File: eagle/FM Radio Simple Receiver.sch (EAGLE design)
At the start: 14 parts, among them T1 2N2222, T2 2N2222

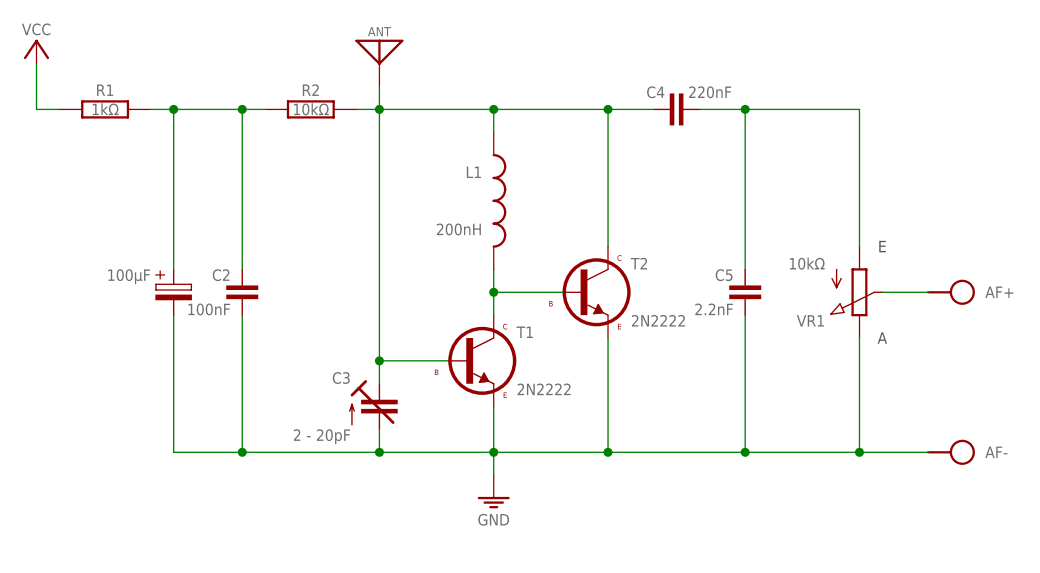
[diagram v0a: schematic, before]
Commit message: ...
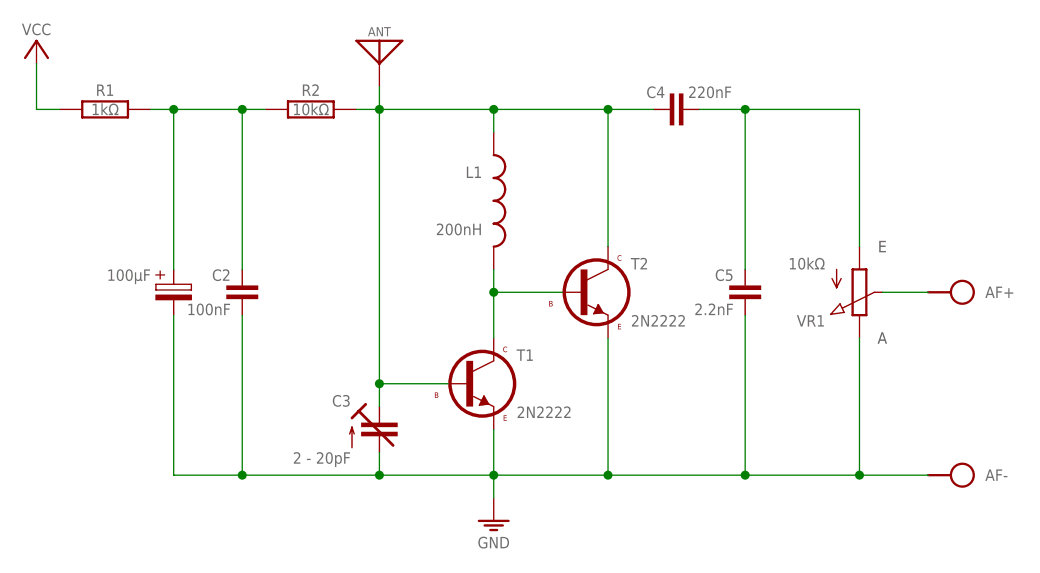
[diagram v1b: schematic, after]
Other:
- moved on the sheet: AF-, C3, T1
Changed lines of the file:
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@@
 </plain>
 <instances>
-<instance part="T1" gate="G$1" x="38.1" y="60.96"/>
-<instance part="C3" gate="1" x="27.94" y="55.88"/>
+<instance part="T1" gate="G$1" x="38.1" y="58.42"/>
+<instance part="C3" gate="1" x="27.94" y="53.34"/>
 <instance part="L1" gate="1" x="40.64" y="78.74"/>
 <instance part="T2" gate="G$1" x="50.8" y="68.58"/>
@@
 <instance part="VR1" gate="1" x="81.28" y="68.58" rot="MR180"/>
 <instance part="R2" gate="1" x="20.32" y="88.9"/>
-<instance part="AF" gate="-" x="88.9" y="50.8" rot="R180"/>
+<instance part="AF" gate="-" x="88.9" y="48.26" rot="R180"/>
 <instance part="AF" gate="+" x="88.9" y="68.58" rot="R180"/>
 <instance part="BAT" gate="1" x="-10.16" y="93.98"/>
-<instance part="BAT" gate="2" x="40.64" y="48.26"/>
+<instance part="BAT" gate="2" x="40.64" y="45.72"/>
 <instance part="ANT" gate="ANT" x="27.94" y="91.44"/>
 <instance part="C5" gate="1" x="68.58" y="68.58"/>
@@
 <pinref part="C3" gate="1" pin="E"/>
 <pinref part="T1" gate="G$1" pin="B"/>
-<wire x1="35.56" y1="60.96" x2="27.94" y2="60.96" width="0.1524" layer="91"/>
-<wire x1="27.94" y1="60.96" x2="27.94" y2="58.42" width="0.1524" layer="91"/>
-<wire x1="27.94" y1="60.96" x2="27.94" y2="88.9" width="0.1524" layer="91"/>
-<junction x="27.94" y="60.96"/>
+<wire x1="35.56" y1="58.42" x2="27.94" y2="58.42" width="0.1524" layer="91"/>
+<wire x1="27.94" y1="58.42" x2="27.94" y2="55.88" width="0.1524" layer="91"/>
+<wire x1="27.94" y1="58.42" x2="27.94" y2="88.9" width="0.1524" layer="91"/>
+<junction x="27.94" y="58.42"/>
 <pinref part="C4" gate="1" pin="1"/>
 <pinref part="L1" gate="1" pin="1"/>
@@
 <wire x1="40.64" y1="71.12" x2="40.64" y2="68.58" width="0.1524" layer="91"/>
 <pinref part="T2" gate="G$1" pin="B"/>
-<wire x1="40.64" y1="68.58" x2="40.64" y2="66.04" width="0.1524" layer="91"/>
+<wire x1="40.64" y1="68.58" x2="40.64" y2="63.5" width="0.1524" layer="91"/>
 <wire x1="48.26" y1="68.58" x2="40.64" y2="68.58" width="0.1524" layer="91"/>
 <junction x="40.64" y="68.58"/>
@@
 <segment>
 <pinref part="BAT" gate="2" pin="GND"/>
-<wire x1="40.64" y1="50.8" x2="40.64" y2="48.26" width="0.1524" layer="91"/>
+<wire x1="40.64" y1="48.26" x2="40.64" y2="45.72" width="0.1524" layer="91"/>
 <pinref part="VR1" gate="1" pin="E"/>
-<wire x1="81.28" y1="50.8" x2="81.28" y2="63.5" width="0.1524" layer="91"/>
+<wire x1="81.28" y1="48.26" x2="81.28" y2="63.5" width="0.1524" layer="91"/>
 <pinref part="AF" gate="-" pin="P$1"/>
-<wire x1="88.9" y1="50.8" x2="81.28" y2="50.8" width="0.1524" layer="91"/>
+<wire x1="88.9" y1="48.26" x2="81.28" y2="48.26" width="0.1524" layer="91"/>
 <pinref part="T1" gate="G$1" pin="E"/>
-<wire x1="40.64" y1="55.88" x2="40.64" y2="50.8" width="0.1524" layer="91"/>
-<wire x1="40.64" y1="50.8" x2="53.34" y2="50.8" width="0.1524" layer="91"/>
-<junction x="81.28" y="50.8"/>
+<wire x1="40.64" y1="53.34" x2="40.64" y2="48.26" width="0.1524" layer="91"/>
+<wire x1="40.64" y1="48.26" x2="53.34" y2="48.26" width="0.1524" layer="91"/>
+<junction x="81.28" y="48.26"/>
 <pinref part="T2" gate="G$1" pin="E"/>
-<wire x1="53.34" y1="50.8" x2="68.58" y2="50.8" width="0.1524" layer="91"/>
-<wire x1="68.58" y1="50.8" x2="81.28" y2="50.8" width="0.1524" layer="91"/>
-<wire x1="53.34" y1="63.5" x2="53.34" y2="50.8" width="0.1524" layer="91"/>
-<junction x="53.34" y="50.8"/>
+<wire x1="53.34" y1="48.26" x2="68.58" y2="48.26" width="0.1524" layer="91"/>
+<wire x1="68.58" y1="48.26" x2="81.28" y2="48.26" width="0.1524" layer="91"/>
+<wire x1="53.34" y1="63.5" x2="53.34" y2="48.26" width="0.1524" layer="91"/>
+<junction x="53.34" y="48.26"/>
 <pinref part="C5" gate="1" pin="2"/>
-<wire x1="68.58" y1="66.04" x2="68.58" y2="50.8" width="0.1524" layer="91"/>
-<junction x="68.58" y="50.8"/>
-<junction x="40.64" y="50.8"/>
+<wire x1="68.58" y1="66.04" x2="68.58" y2="48.26" width="0.1524" layer="91"/>
+<junction x="68.58" y="48.26"/>
+<junction x="40.64" y="48.26"/>
 <pinref part="C3" gate="1" pin="A"/>
-<wire x1="27.94" y1="53.34" x2="27.94" y2="50.8" width="0.1524" layer="91"/>
-<wire x1="27.94" y1="50.8" x2="40.64" y2="50.8" width="0.1524" layer="91"/>
-<wire x1="27.94" y1="50.8" x2="12.7" y2="50.8" width="0.1524" layer="91"/>
-<junction x="27.94" y="50.8"/>
+<wire x1="27.94" y1="50.8" x2="27.94" y2="48.26" width="0.1524" layer="91"/>
+<wire x1="27.94" y1="48.26" x2="40.64" y2="48.26" width="0.1524" layer="91"/>
+<wire x1="27.94" y1="48.26" x2="12.7" y2="48.26" width="0.1524" layer="91"/>
+<junction x="27.94" y="48.26"/>
 <pinref part="C2" gate="1" pin="2"/>
-<wire x1="12.7" y1="50.8" x2="12.7" y2="66.04" width="0.1524" layer="91"/>
+<wire x1="12.7" y1="48.26" x2="12.7" y2="66.04" width="0.1524" layer="91"/>
 <pinref part="100µF" gate="1" pin="-"/>
-<wire x1="5.08" y1="66.04" x2="5.08" y2="50.8" width="0.1524" layer="91"/>
-<wire x1="5.08" y1="50.8" x2="12.7" y2="50.8" width="0.1524" layer="91"/>
-<junction x="12.7" y="50.8"/>
+<wire x1="5.08" y1="66.04" x2="5.08" y2="48.26" width="0.1524" layer="91"/>
+<wire x1="5.08" y1="48.26" x2="12.7" y2="48.26" width="0.1524" layer="91"/>
+<junction x="12.7" y="48.26"/>
 </segment>
 </net>
